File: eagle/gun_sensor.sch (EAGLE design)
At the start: 17 parts, among them IC2 AD823, IC3 LM328

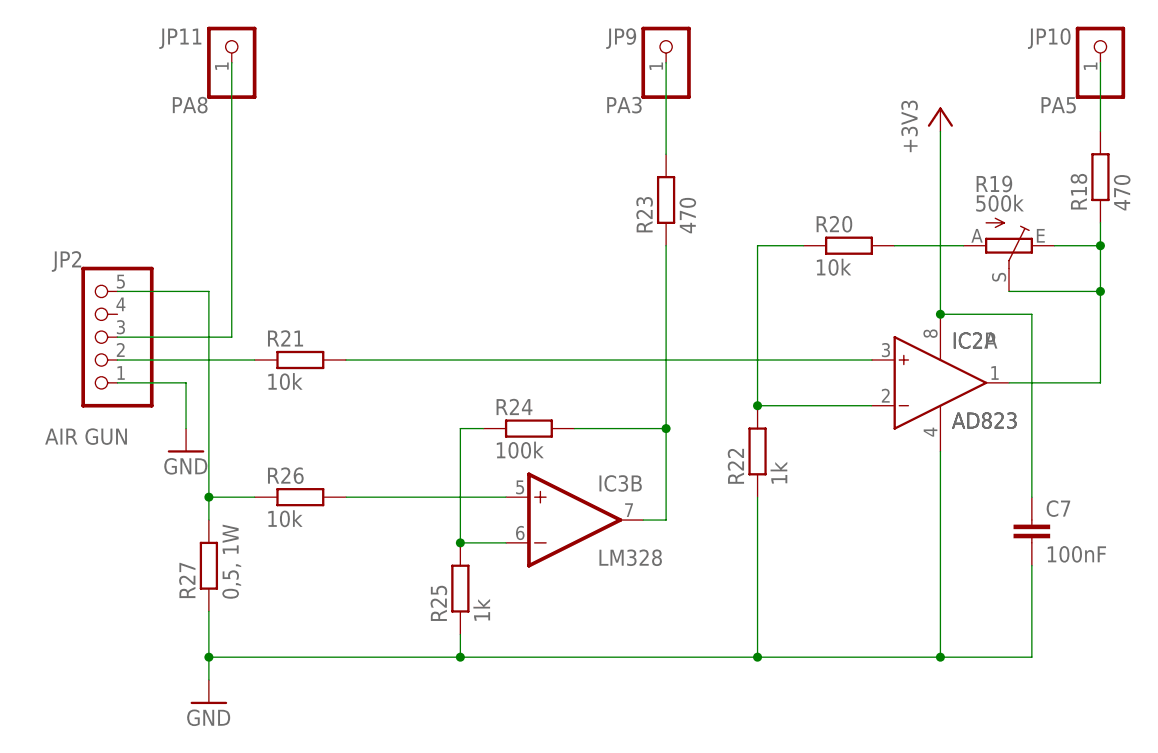
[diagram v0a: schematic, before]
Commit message: Add files via upload
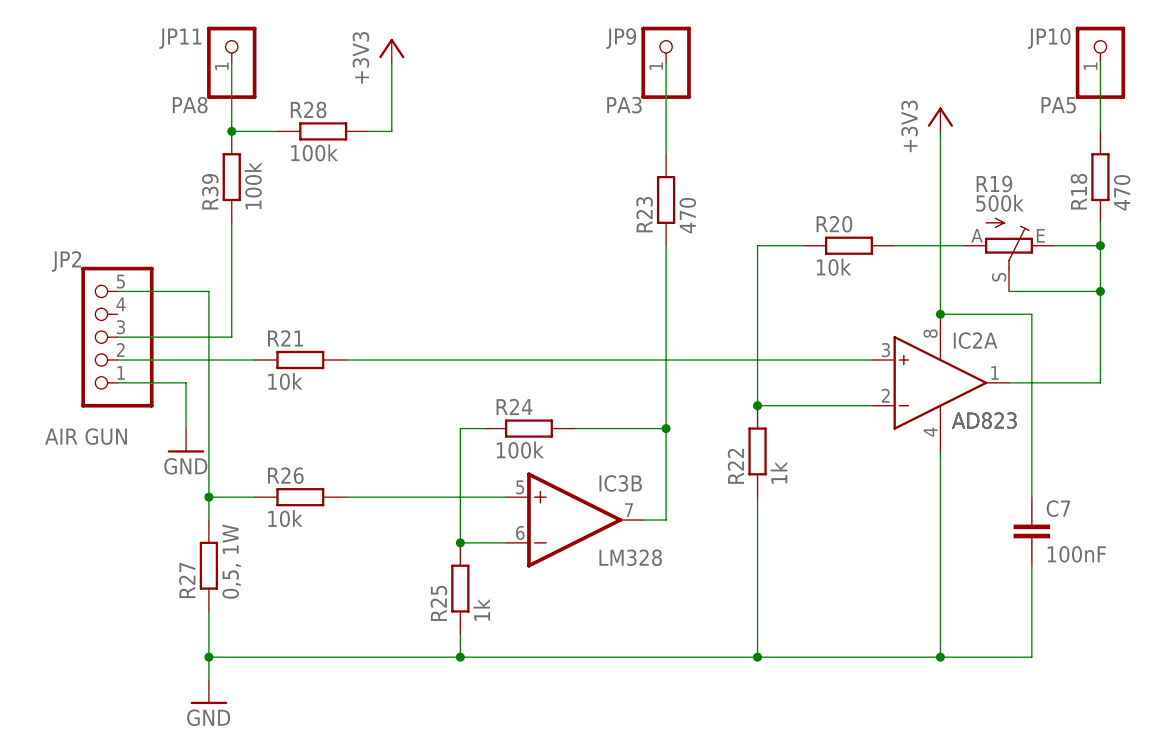
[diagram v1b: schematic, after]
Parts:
- added R28, R39: 100k, rcl:R-EU_0204/5
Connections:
- new net N$13: JP11.1, R28.1, R39.2
- net +3V3: now also R28.2
- net N$7: now also R39.1; no longer JP11.1
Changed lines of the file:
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@@
 <?xml version="1.0" encoding="utf-8"?>
 <!DOCTYPE eagle SYSTEM "eagle.dtd">
-<eagle version="9.2.0">
+<eagle version="9.2.2">
 <drawing>
 <settings>
@@
 <part name="IC3" library="linear" library_urn="urn:adsk.eagle:library:262" deviceset="MCP602" device="P" package3d_urn="urn:adsk.eagle:package:16409/2" value="LM328"/>
 <part name="C7" library="rcl" library_urn="urn:adsk.eagle:library:334" deviceset="C-EU" device="025-024X044" package3d_urn="urn:adsk.eagle:package:23630/1" value="100nF"/>
+<part name="R39" library="rcl" library_urn="urn:adsk.eagle:library:334" deviceset="R-EU_" device="0204/5" package3d_urn="urn:adsk.eagle:package:23488/1" value="100k"/>
+<part name="R28" library="rcl" library_urn="urn:adsk.eagle:library:334" deviceset="R-EU_" device="0204/5" package3d_urn="urn:adsk.eagle:package:23488/1" value="100k"/>
+<part name="+3V2" library="supply1" library_urn="urn:adsk.eagle:library:371" deviceset="+3V3" device=""/>
 </parts>
 <sheets>
@@
 </plain>
 <instances>
-<instance part="R27" gate="G$1" x="-17.78" y="20.32" rot="R90">
+<instance part="R27" gate="G$1" x="-17.78" y="20.32" smashed="yes" rot="R90">
 <attribute name="NAME" x="-19.2786" y="16.51" size="1.778" layer="95" rot="R90"/>
 <attribute name="VALUE" x="-14.478" y="16.51" size="1.778" layer="96" rot="R90"/>
 </instance>
-<instance part="IC2" gate="A" x="60.96" y="40.64">
+<instance part="IC2" gate="A" x="60.96" y="40.64" smashed="yes">
 <attribute name="NAME" x="64.77" y="44.45" size="1.778" layer="95"/>
 <attribute name="VALUE" x="64.77" y="35.56" size="1.778" layer="96"/>
 </instance>
-<instance part="IC2" gate="P" x="63.5" y="40.64">
+<instance part="IC2" gate="P" x="63.5" y="40.64" smashed="yes">
 <attribute name="VALUE" x="64.77" y="35.56" size="1.778" layer="96"/>
 </instance>
-<instance part="R26" gate="G$1" x="-7.62" y="27.94">
+<instance part="R26" gate="G$1" x="-7.62" y="27.94" smashed="yes">
 <attribute name="NAME" x="-11.43" y="29.4386" size="1.778" layer="95"/>
 <attribute name="VALUE" x="-11.43" y="24.638" size="1.778" layer="96"/>
 </instance>
-<instance part="GND1" gate="1" x="-17.78" y="5.08">
+<instance part="GND1" gate="1" x="-17.78" y="5.08" smashed="yes">
 <attribute name="VALUE" x="-20.32" y="2.54" size="1.778" layer="96"/>
 </instance>
-<instance part="R25" gate="G$1" x="10.16" y="17.78" rot="R90">
+<instance part="R25" gate="G$1" x="10.16" y="17.78" smashed="yes" rot="R90">
 <attribute name="NAME" x="8.6614" y="13.97" size="1.778" layer="95" rot="R90"/>
 <attribute name="VALUE" x="13.462" y="13.97" size="1.778" layer="96" rot="R90"/>
 </instance>
-<instance part="R24" gate="G$1" x="17.78" y="35.56">
+<instance part="R24" gate="G$1" x="17.78" y="35.56" smashed="yes">
 <attribute name="NAME" x="13.97" y="37.0586" size="1.778" layer="95"/>
 <attribute name="VALUE" x="13.97" y="32.258" size="1.778" layer="96"/>
 </instance>
-<instance part="R22" gate="G$1" x="43.18" y="33.02" rot="R90">
+<instance part="R22" gate="G$1" x="43.18" y="33.02" smashed="yes" rot="R90">
 <attribute name="NAME" x="41.6814" y="29.21" size="1.778" layer="95" rot="R90"/>
 <attribute name="VALUE" x="46.482" y="29.21" size="1.778" layer="96" rot="R90"/>
 </instance>
-<instance part="R21" gate="G$1" x="-7.62" y="43.18">
+<instance part="R21" gate="G$1" x="-7.62" y="43.18" smashed="yes">
 <attribute name="NAME" x="-11.43" y="44.6786" size="1.778" layer="95"/>
 <attribute name="VALUE" x="-11.43" y="39.878" size="1.778" layer="96"/>
 </instance>
-<instance part="R19" gate="1" x="71.12" y="55.88" rot="R270">
+<instance part="R19" gate="1" x="71.12" y="55.88" smashed="yes" rot="R270">
 <attribute name="NAME" x="67.31" y="61.849" size="1.778" layer="95"/>
 <attribute name="VALUE" x="67.31" y="59.69" size="1.778" layer="96"/>
 </instance>
-<instance part="R20" gate="G$1" x="53.34" y="55.88">
+<instance part="R20" gate="G$1" x="53.34" y="55.88" smashed="yes">
 <attribute name="NAME" x="49.53" y="57.3786" size="1.778" layer="95"/>
 <attribute name="VALUE" x="49.53" y="52.578" size="1.778" layer="96"/>
 </instance>
-<instance part="R23" gate="G$1" x="33.02" y="60.96" rot="R90">
+<instance part="R23" gate="G$1" x="33.02" y="60.96" smashed="yes" rot="R90">
 <attribute name="NAME" x="31.5214" y="57.15" size="1.778" layer="95" rot="R90"/>
 <attribute name="VALUE" x="36.322" y="57.15" size="1.778" layer="96" rot="R90"/>
 </instance>
-<instance part="JP9" gate="G$1" x="33.02" y="78.74" rot="R90">
+<instance part="JP9" gate="G$1" x="33.02" y="78.74" smashed="yes" rot="R90">
 <attribute name="NAME" x="29.845" y="80.01" size="1.778" layer="95" rot="R180"/>
 <attribute name="VALUE" x="30.48" y="72.39" size="1.778" layer="96" rot="R180"/>
 </instance>
-<instance part="R18" gate="G$1" x="81.28" y="63.5" rot="R90">
+<instance part="R18" gate="G$1" x="81.28" y="63.5" smashed="yes" rot="R90">
 <attribute name="NAME" x="79.7814" y="59.69" size="1.778" layer="95" rot="R90"/>
 <attribute name="VALUE" x="84.582" y="59.69" size="1.778" layer="96" rot="R90"/>
 </instance>
-<instance part="JP10" gate="G$1" x="81.28" y="78.74" rot="R90">
+<instance part="JP10" gate="G$1" x="81.28" y="78.74" smashed="yes" rot="R90">
 <attribute name="NAME" x="78.105" y="80.01" size="1.778" layer="95" rot="R180"/>
 <attribute name="VALUE" x="78.74" y="72.39" size="1.778" layer="96" rot="R180"/>
 </instance>
-<instance part="+3V1" gate="G$1" x="63.5" y="71.12">
+<instance part="+3V1" gate="G$1" x="63.5" y="71.12" smashed="yes">
 <attribute name="VALUE" x="60.96" y="66.04" size="1.778" layer="96" rot="R90"/>
 </instance>
-<instance part="JP2" gate="A" x="-30.48" y="45.72" rot="R180">
+<instance part="JP2" gate="A" x="-30.48" y="45.72" smashed="yes" rot="R180">
 <attribute name="NAME" x="-31.75" y="55.245" size="1.778" layer="95" rot="R180"/>
 <attribute name="VALUE" x="-26.67" y="35.56" size="1.778" layer="96" rot="R180"/>
 </instance>
-<instance part="GND2" gate="1" x="-20.32" y="33.02">
+<instance part="GND2" gate="1" x="-20.32" y="33.02" smashed="yes">
 <attribute name="VALUE" x="-22.86" y="30.48" size="1.778" layer="96"/>
 </instance>
-<instance part="JP11" gate="G$1" x="-15.24" y="78.74" rot="R90">
+<instance part="JP11" gate="G$1" x="-15.24" y="78.74" smashed="yes" rot="R90">
 <attribute name="NAME" x="-18.415" y="80.01" size="1.778" layer="95" rot="R180"/>
 <attribute name="VALUE" x="-17.78" y="72.39" size="1.778" layer="96" rot="R180"/>
 </instance>
-<instance part="IC3" gate="B" x="22.86" y="25.4">
+<instance part="IC3" gate="B" x="22.86" y="25.4" smashed="yes">
 <attribute name="NAME" x="25.4" y="28.575" size="1.778" layer="95"/>
 <attribute name="VALUE" x="25.4" y="20.32" size="1.778" layer="96"/>
 </instance>
-<instance part="C7" gate="G$1" x="73.66" y="25.4">
+<instance part="C7" gate="G$1" x="73.66" y="25.4" smashed="yes">
 <attribute name="NAME" x="75.184" y="25.781" size="1.778" layer="95"/>
 <attribute name="VALUE" x="75.184" y="20.701" size="1.778" layer="96"/>
+</instance>
+<instance part="R39" gate="G$1" x="-15.24" y="63.5" smashed="yes" rot="R90">
+<attribute name="NAME" x="-16.7386" y="59.69" size="1.778" layer="95" rot="R90"/>
+<attribute name="VALUE" x="-11.938" y="59.69" size="1.778" layer="96" rot="R90"/>
+</instance>
+<instance part="R28" gate="G$1" x="-5.08" y="68.58" smashed="yes">
+<attribute name="NAME" x="-8.89" y="70.0786" size="1.778" layer="95"/>
+<attribute name="VALUE" x="-8.89" y="65.278" size="1.778" layer="96"/>
+</instance>
+<instance part="+3V2" gate="G$1" x="2.54" y="78.74" smashed="yes">
+<attribute name="VALUE" x="0" y="73.66" size="1.778" layer="96" rot="R90"/>
 </instance>
 </instances>
@@
 <junction x="63.5" y="48.26"/>
 </segment>
+<segment>
+<pinref part="+3V2" gate="G$1" pin="+3V3"/>
+<wire x1="2.54" y1="76.2" x2="2.54" y2="68.58" width="0.1524" layer="91"/>
+<pinref part="R28" gate="G$1" pin="2"/>
+<wire x1="2.54" y1="68.58" x2="0" y2="68.58" width="0.1524" layer="91"/>
+</segment>
 </net>
 <net name="N$10" class="0">
@@
 <pinref part="JP2" gate="A" pin="3"/>
 <wire x1="-27.94" y1="45.72" x2="-15.24" y2="45.72" width="0.1524" layer="91"/>
-<wire x1="-15.24" y1="45.72" x2="-15.24" y2="76.2" width="0.1524" layer="91"/>
+<pinref part="R39" gate="G$1" pin="1"/>
+<wire x1="-15.24" y1="58.42" x2="-15.24" y2="45.72" width="0.1524" layer="91"/>
+</segment>
+</net>
+<net name="N$13" class="0">
+<segment>
+<pinref part="R28" gate="G$1" pin="1"/>
+<pinref part="R39" gate="G$1" pin="2"/>
+<wire x1="-10.16" y1="68.58" x2="-15.24" y2="68.58" width="0.1524" layer="91"/>
 <pinref part="JP11" gate="G$1" pin="1"/>
-</segment>
-</net>
+<wire x1="-15.24" y1="68.58" x2="-15.24" y2="76.2" width="0.1524" layer="91"/>
+<junction x="-15.24" y="68.58"/>
+</segment>
+</net>
